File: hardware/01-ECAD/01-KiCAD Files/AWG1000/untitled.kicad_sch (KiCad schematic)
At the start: 4 parts

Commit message: Update.
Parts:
- removed U? (x4): XC7A35T-1CSG325C, CSG324_ARTIX_XIL, symbol awg1000:XC7A35T-1CSG325C
- added U36: LFE3-35EA-7FN484I, Package_BGA:BGA-484_23.0x23.0mm_Layout22x22_P1.0mm, symbol awg1000:LFE3-35EA-7FN484I
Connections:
- new net: U36.H14 (VCCIO1), U36.H16 (VCCIO8), U36.J15 (VCCIO2)
- new net: U36.J10 (VCC), U36.J11 (VCC), U36.J12 (VCC), U36.J13 (VCC), U36.J14 (VCC)
- new net: U36.N16 (VCCIO3), U36.P10 (VCC), U36.P11 (VCC), U36.P12 (VCC), U36.P13 (VCC), U36.P14 (VCC)
- new net: U36.U11 (VCCA), U36.U12 (VCCA), U36.V10 (VCCA), U36.V13 (VCCA)
- new net: U36.H9 (VCCIO0), U36.J8 (VCCIO7)
- new net: U36.L9 (VCC), U36.P9 (VCC)
- new net: U36.G13 (VCCIO1), U36.G16 (VCCIO8)
- new net GND: U36.A1 (GND), U36.A22 (GND), U36.AA10 (GND), U36.AA11 (GND), U36.AA12 (GND), U36.AA13 (GND), U36.AA14 (GND), U36.AA15 (GND), U36.AA16 (GND), U36.AA18 (GND), U36.AA9 (GND), U36.AB16 (GND), U36.AB22 (GND), U36.B13 (GND), U36.B17 (GND), U36.B5 (GND), U36.B9 (GND), U36.C11 (GND), U36.C19 (GND), U36.C4 (TMS), U36.D3 (GND), U36.E21 (GND), U36.E8 (GND), U36.F17 (GND), U36.F2 (GND), U36.F6 (GND), U36.G11 (GND), U36.G12 (GND), U36.H10 (GND), U36.H15 (GND), U36.H8 (GND), U36.J21 (GND), U36.J5 (GND), U36.K10 (GND), U36.K11 (GND), U36.K12 (GND), U36.K13 (GND), U36.K15 (GND), U36.K2 (GND), U36.K8 (GND), U36.L10 (GND), U36.L11 (GND), U36.L12 (GND), U36.L13 (GND), U36.L20 (GND), U36.L7 (GND), U36.M10 (GND), U36.M11 (GND), U36.M12 (GND), U36.M13 (GND), U36.M16 (GND), U36.N10 (GND), U36.N11 (GND), U36.N12 (GND), U36.N13 (GND), U36.N21 (GND), U36.N8 (GND), U36.P16 (GND), U36.P18 (GND), U36.P2 (GND), U36.R13 (GND), U36.R15 (GND), U36.R5 (GND), U36.R8 (GND), U36.T13 (GND), U36.U13 (GND), U36.U14 (GND), U36.U17 (GND), U36.U21 (GND), U36.U6 (GND), U36.U9 (GND), U36.V14 (GND), U36.V15 (GND), U36.V16 (GND), U36.V2 (GND), U36.V7 (GND), U36.V8 (GND), U36.V9 (GND), U36.W16 (GND), U36.W20 (GND), U36.W7 (GND), U36.Y16 (GND), U36.Y4 (GND), U36.Y7 (GND)

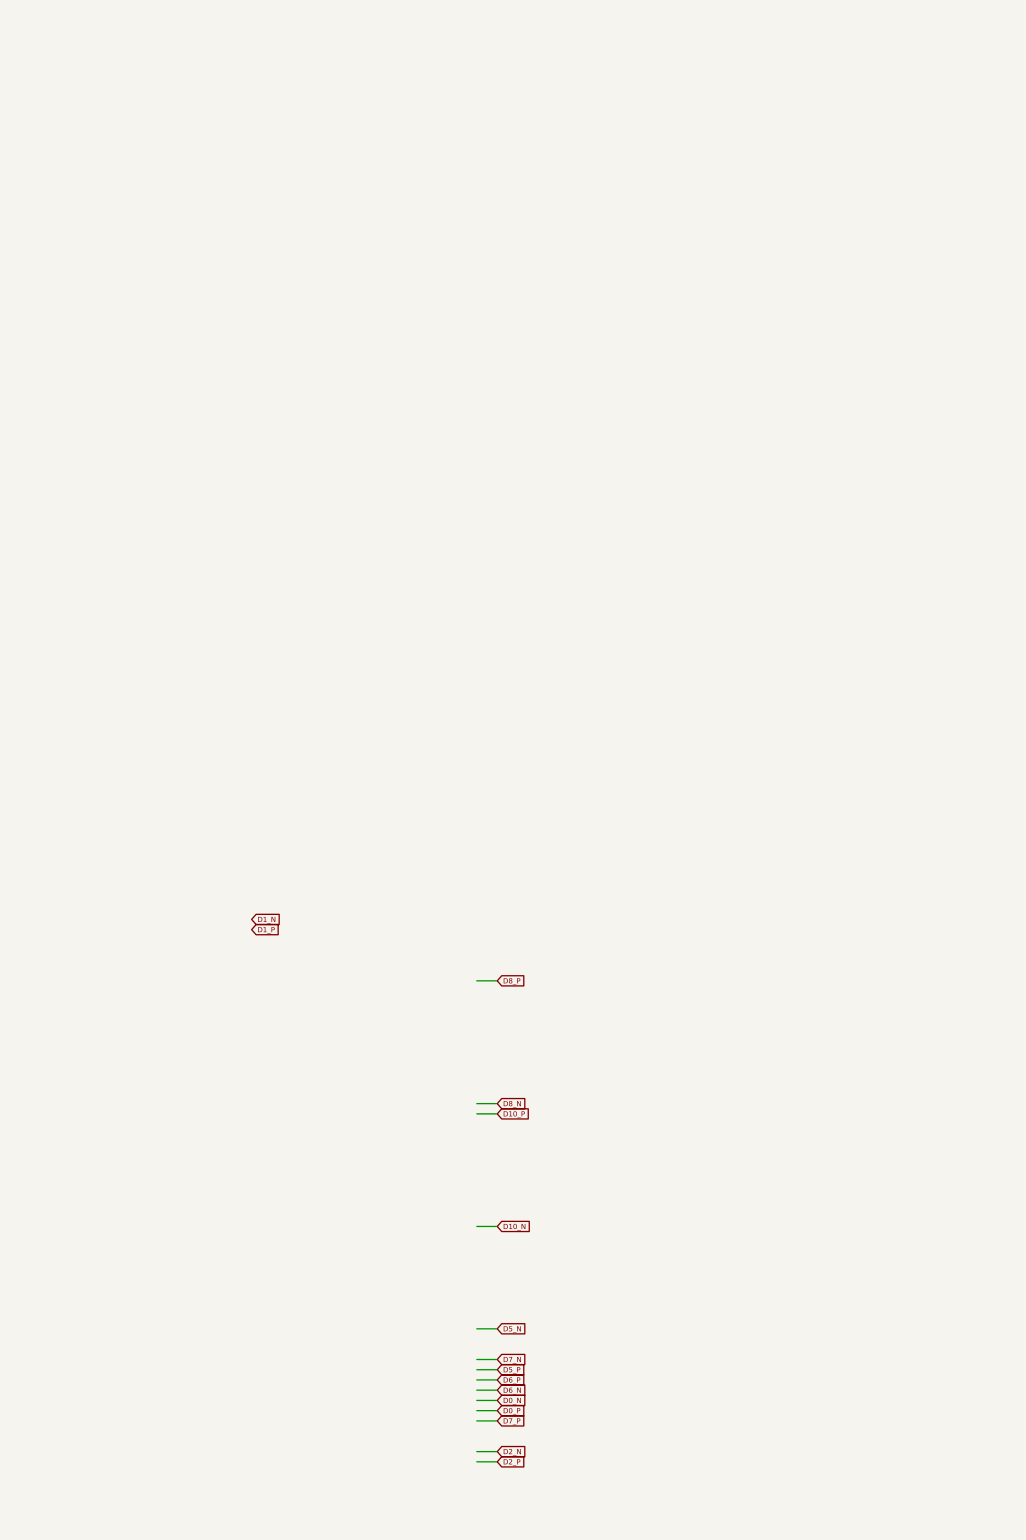
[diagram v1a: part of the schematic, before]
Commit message: Update.
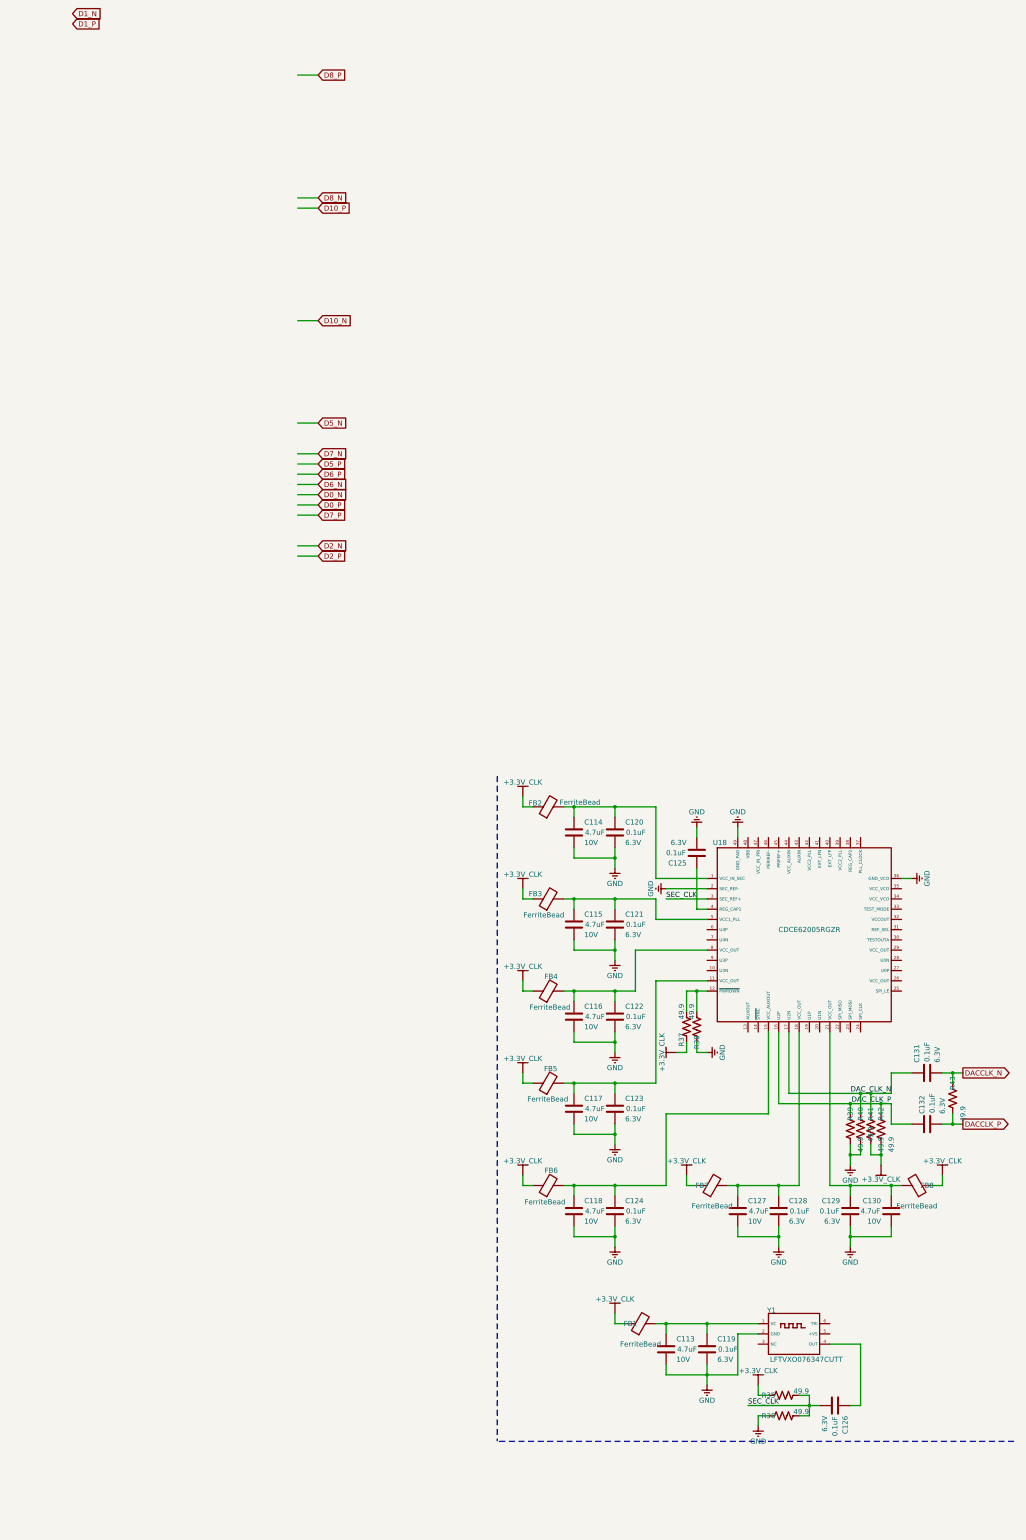
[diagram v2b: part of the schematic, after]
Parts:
- added C113, C114, C115, C116, C117, C118, C127, C130: 4.7uF, awg1000:C0402_L, symbol Device:C
- added C119, C120, C121, C122, C123, C124, C125, C126, C128, C129, C131, C132: 0.1uF, Resistor_SMD:R_0402_1005Metric_Pad0.72x0.64mm_HandSolder, symbol Device:C
- added FB1, FB2, FB3, FB4, FB5, FB6, FB7, FB8: FerriteBead, Inductor_SMD:L_0402_1005Metric_Pad0.77x0.64mm_HandSolder, symbol Device:FerriteBead
- added R35, R36, R37, R38, R39, R40, R41, R42, R43: 49.9, Resistor_SMD:R_0402_1005Metric_Pad0.72x0.64mm_HandSolder, symbol Device:R_US
- added U18: CDCE62005RGZR, Package_DFN_QFN:QFN-48-1EP_7x7mm_P0.5mm_EP5.6x5.6mm_ThermalVias, symbol awg1000:CDCE62005RGZR
- added Y1: LFTVXO076347CUTT, awg1000:IQXT-316-5, symbol awg1000:LFTVXO076347CUTT
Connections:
- net DACCLK_N: now also C131.2, R43.2
- net DACCLK_P: now also C132.2, R43.1
- net GND: now also C113.2, C114.2, C115.2, C116.2, C117.2, C118.2, C119.2, C120.2, C121.2, C122.2, C123.2, C124.2, C125.2, C127.2, C128.2, C129.2, C130.2, R36.2, R38.2, R39.1, R40.1, U18.2 (SEC_REF-), U18.36 (GND_VCO), U18.49 (GND_PAD), Y1.2 (GND)
- new net: C118.1, C124.1, FB6.2, U18.15 (VCC_AUXOUT)
- new net: C114.1, C120.1, FB2.2, U18.1 (VCC_IN_SEC)
- new net: R37.1, R38.1, U18.12 (~{PWRDWN})
- new net: C116.1, C122.1, FB4.2, U18.8 (VCC_OUT)
- new net: C113.1, C119.1, FB1.2, Y1.1 (VC)
- new net: C115.1, C121.1, FB3.2, U18.5 (VCC1_PLL)
- new net: C129.1, C130.1, FB8.2, U18.21 (VCC_OUT)
- new net: C127.1, C128.1, FB7.2, U18.18 (VCC_OUT)
- new net: C125.1, U18.4 (REG_CAP1)
- new net: C117.1, C123.1, FB5.2, U18.11 (VCC_OUT)
- new net: C126.1, Y1.4 (OUT)
- new net +3.3V_CLK: FB1.1, FB2.1, FB3.1, FB4.1, FB5.1, FB6.1, FB7.1, FB8.1, R35.2, R37.2, R41.1, R42.1
- new net DAC_CLK_N: C131.1, R40.2, R41.2, U18.17 (U2N)
- new net DAC_CLK_P: C132.1, R39.2, R42.2, U18.16 (U2P)
- new net SEC_CLK: C126.2, R35.1, R36.1, U18.3 (SEC_REF+)

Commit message: Update.
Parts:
- added C385, C386, C387, C388: 0.1uF, Resistor_SMD:R_0402_1005Metric_Pad0.72x0.64mm_HandSolder, symbol awg1000:CAP_UNPOL
- added R161, R162, R163, R164, R165, R166, R167, R168, R169, R170, R171, R172, R173: 49.9, Resistor_SMD:R_0402_1005Metric_Pad0.72x0.64mm_HandSolder, symbol awg1000:R
- C113, C114, C115, C116, C117, C118, C127, C130: footprint awg1000:C0402_L -> Capacitor_SMD:C_0402_1005Metric_Pad0.74x0.62mm_HandSolder; symbol Device:C -> awg1000:CAP_UNPOL; Part Number C1005X5R1A475K050BE -> (none)
- C119, C120, C121, C122, C123, C124, C125, C126, C128, C129, C131, C132: symbol Device:C -> awg1000:CAP_UNPOL
- R35, R36, R37, R38, R39, R40, R41, R42, R43: symbol Device:R_US -> awg1000:R
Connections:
- net +3.3V_CLK: now also R39.2, R42.2, U18.10 (U3N), C385.1, R162.2, R163.1, R163.2, R164.1, R169.2, R170.2; no longer R41.1, R42.1
- net D0_N: now also U36.E4 (PL11B)
- net D0_P: now also U36.E5 (PL11A)
- net D10_N: now also U36.R1 (PL48B)
- net D10_P: now also U36.P1 (PL48A)
- net D11_N: now also U36.U2 (PL53B)
- net D11_P: now also U36.U1 (PL53A)
- net D12_N: now also U36.U4 (PL65B)
- net D12_P: now also U36.T4 (PL65A)
- net D13_N: now also U36.Y2 (PL66B)
- net D13_P: now also U36.AA1 (PL66A)
- net D14_N: now also U36.V5 (PL71B)
- net D14_P: now also U36.V4 (PL71A)
- net D15_P: now also U36.H2 (PL30A), U36.H3 (PL30B)
- net D1_N: now also U36.C2 (PL12B)
- net D1_P: now also U36.B2 (PL12A)
- net D2_N: now also U36.G5 (PL17B)
- net D2_P: now also U36.G4 (PL17A)
- net D3_N: now also U36.J4 (PL20B)
- net D3_P: now also U36.H4 (PL20A)
- net D4_N: now also U36.C1 (PL21B)
- net D4_P: now also U36.B1 (PL21A)
- net D5_N: now also U36.F1 (PL26B)
- net D5_P: now also U36.E1 (PL26A)
- net D6_N: now also U36.M4 (PL38B)
- net D6_P: now also U36.L4 (PL38A)
- net D7_N: now also U36.M1 (PL39B)
- net D7_P: now also U36.M2 (PL39A)
- net D8_N: now also U36.P4 (PL44B)
- net D8_P: now also U36.N4 (PL44A)
- net D9_N: now also U36.P6 (PL47B)
- net D9_P: now also U36.N5 (PL47A)
- net DACCLK_N: now also R43.1; no longer R43.2
- net DACCLK_P: now also R43.2; no longer R43.1
- net DAC_CLK_N: now also R41.1, R42.1, U18.16 (U2P); no longer R40.2, R41.2, U18.17 (U2N)
- net DAC_CLK_P: now also R39.1, R40.1, U18.17 (U2N); no longer R39.2, R42.2, U18.16 (U2P)
- net GND: now also C125.1, R40.2, R41.2, U18.43 (AUXIN), R164.2, R165.2, R171.2, R172.2; no longer C125.2, R39.1, R40.1
- net SYNC_N: now also U36.W1 (PL57B)
- net SYNC_P: now also U36.V1 (PL57A)
- net 1.2V_DAC_DVDD: now reaches U36.J10 (VCC), U36.J11 (VCC), U36.J12 (VCC), U36.J13 (VCC), U36.J14 (VCC)
- net 1.2V_DAC_DVDD: now also U36.P10 (VCC), U36.P11 (VCC), U36.P12 (VCC), U36.P13 (VCC), U36.P14 (VCC)
- net FPGACLK_N: now reaches U36.K6 (PL35E_D)
- net FPGACLK_N: now also C385.2, R161.1
- net FPGACLK_P: now reaches U36.P5 (PL50A)
- net FPGACLK_P: now also C386.2, R161.2
- net at U18.4 (REG_CAP1): now also C125.2; no longer C125.1
- net DAC_OSTR_N: now reaches U18.19 (U1P)
- net DAC_OSTR_N: now also C387.1, R170.1, R171.1
- net DAC_OSTR_P: now reaches U18.20 (U1N)
- net DAC_OSTR_P: now also C388.1, R169.1, R172.1
- net CDC-PRIREF+: now reaches U18.45 (PRIFEF+)
- net at U18.46 (PERIREF-): now also R166.1, R167.1, R168.1
- net FPGA_CLK_P: now reaches U18.9 (U3P)
- net FPGA_CLK_P: now also C386.1, R162.1, R165.1
- new net DACOSTR_N: C387.2, R173.1
- new net DACOSTR_P: C388.2, R173.2
- now unconnected: U36.N16 (VCCIO3), U36.U11 (VCCA), U36.U12 (VCCA), U36.V10 (VCCA), U36.V13 (VCCA)
- no-connect marks 0 -> 4
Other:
- note added: "CLOCK GENERATOR"
- moved on the sheet: FB1, FB7, FB8, R35, R36, R39, R40, R41, R42, R43, U36A, U36B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
